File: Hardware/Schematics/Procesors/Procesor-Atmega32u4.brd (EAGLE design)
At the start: 30.5 x 30.1 mm, 5 parts

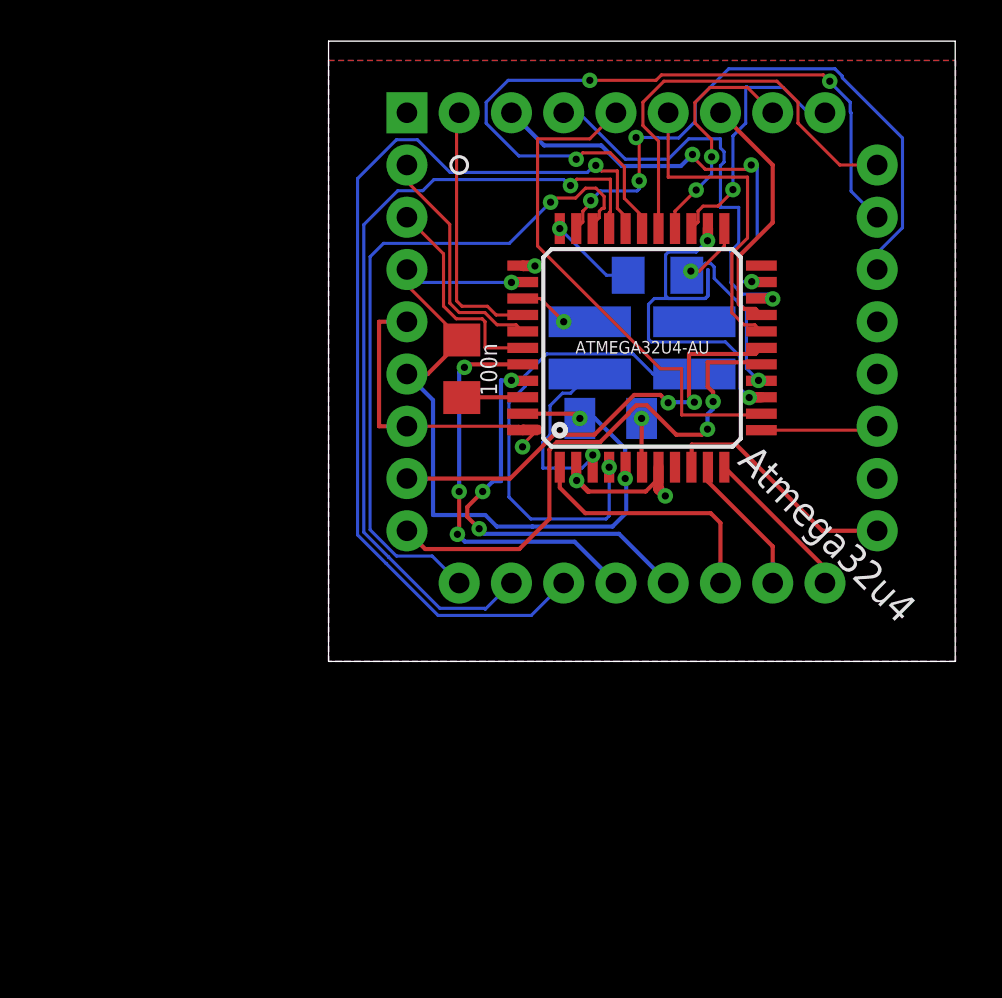
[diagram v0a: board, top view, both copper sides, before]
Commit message: commit
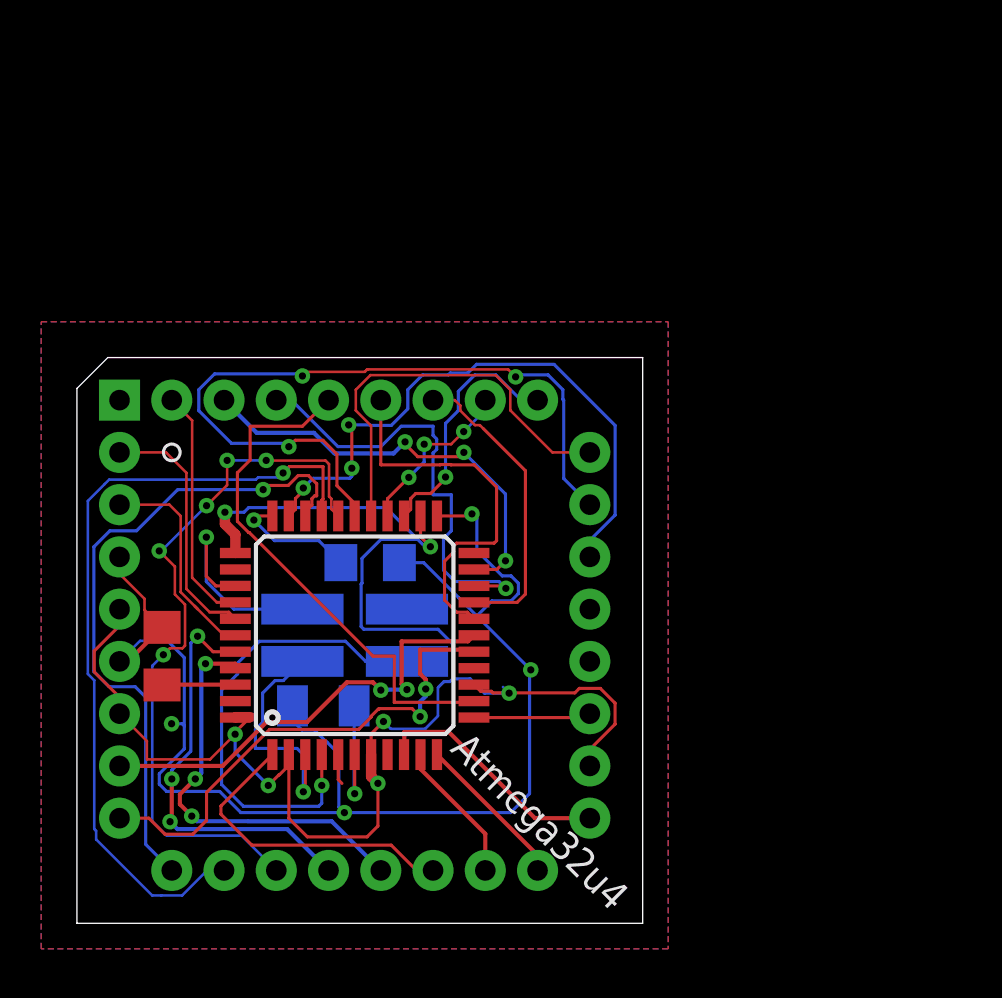
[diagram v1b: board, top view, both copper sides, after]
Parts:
- moved C1 20.2 mm to (-9.36, -1.02)
- moved ATMEGA32U4-AU 19.8 mm to (0.00, 0.00)
- moved R1 19.8 mm to (0.75, 3.53)
- moved U$2 19.8 mm to (0.00, 0.00)
- moved C2 19.8 mm to (-1.52, -3.43)
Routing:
- net +3V3: track 45.9 -> 82.1 mm, vias 6 -> 7
- net GND: track 51.9 -> 69.1 mm, vias 5 -> 4
- net D7: track 46.9 -> 35.3 mm, vias 1 -> 5
- net 36: track 3.73 -> 10.9 mm
- net N$2: track 2.38 -> 6.18 mm
- net A3: track 11.8 -> 8.36 mm, vias 2 -> 3
- net A5: track 15.7 -> 18.6 mm
- net D10: track 12.4 -> 15.4 mm
- net D-: track 9.14 -> 11.5 mm
- net A4: track 12.3 -> 14.7 mm
- net XTAL2: track 26.7 -> 24.6 mm
- net D0: track 20.1 -> 22.2 mm
- net N$6: track 4.27 -> 6.07 mm
- net D5: track 33.4 -> 32.3 mm
- net D2: track 12.7 -> 11.6 mm
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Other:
- board size 30.5 x 30.1 mm -> 27.5 x 27.5 mm
